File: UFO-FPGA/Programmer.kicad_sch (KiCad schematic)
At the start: 42 parts, among them U2 FT2232HL, U3 ASDMB-12MHz, U5 93LC56CT-I/MS

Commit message: pcb
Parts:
- U3: footprint Oscillator:Oscillator_SMD_Abracon_ASDMB-4Pin_2.5x2.0mm -> UFO-Footpints:ASDDV-12.000MHz-LC-T3
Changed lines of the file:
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@@
       (effects (font (size 1.27 1.27)))
     )
-    (property "Footprint" "Oscillator:Oscillator_SMD_Abracon_ASDMB-4Pin_2.5x2.0mm" (at 164.465 185.42 0)
+    (property "Footprint" "UFO-Footpints:ASDDV-12.000MHz-LC-T3" (at 164.465 185.42 0)
       (effects (font (size 1.27 1.27)) hide)
     )

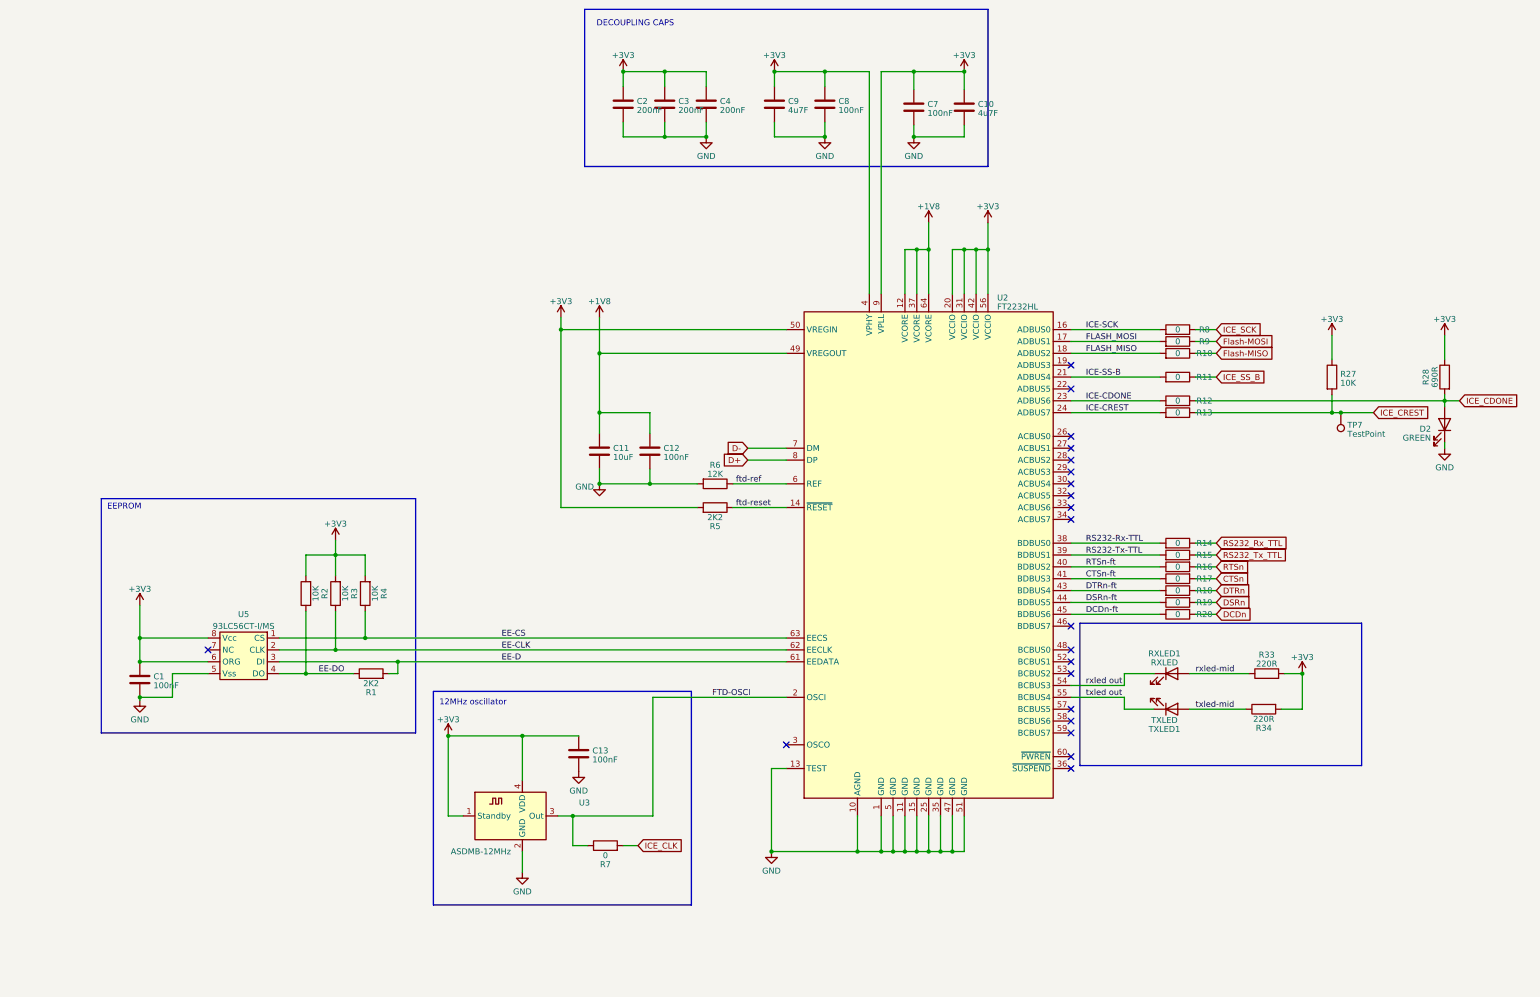
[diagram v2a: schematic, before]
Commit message: schema
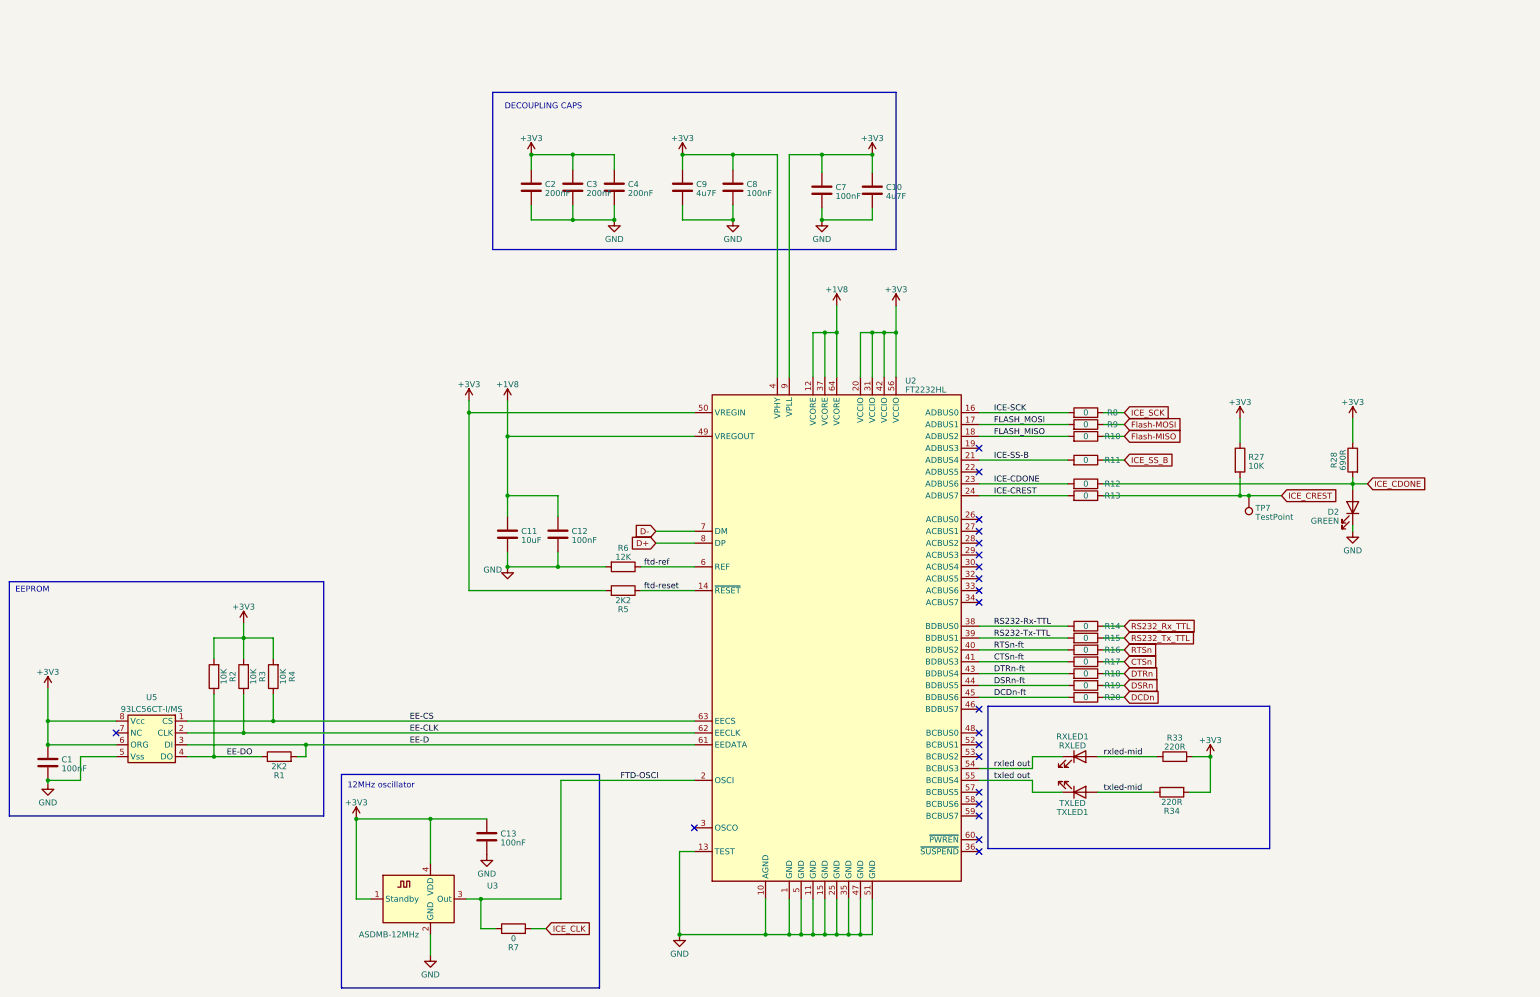
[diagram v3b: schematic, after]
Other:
- title: (none) -> FT2232H usb prog
- moved on the sheet: C1, C10, C11, C12, C13, C2, C3, C4, C7, C8, C9, D2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
